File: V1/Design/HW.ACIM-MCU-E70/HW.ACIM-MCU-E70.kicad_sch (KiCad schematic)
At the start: 35 parts, among them J1 HEADER 2x15POS, J2 HEADER 2x15POS, U1 ATSAME70J20B, U2 12MHz

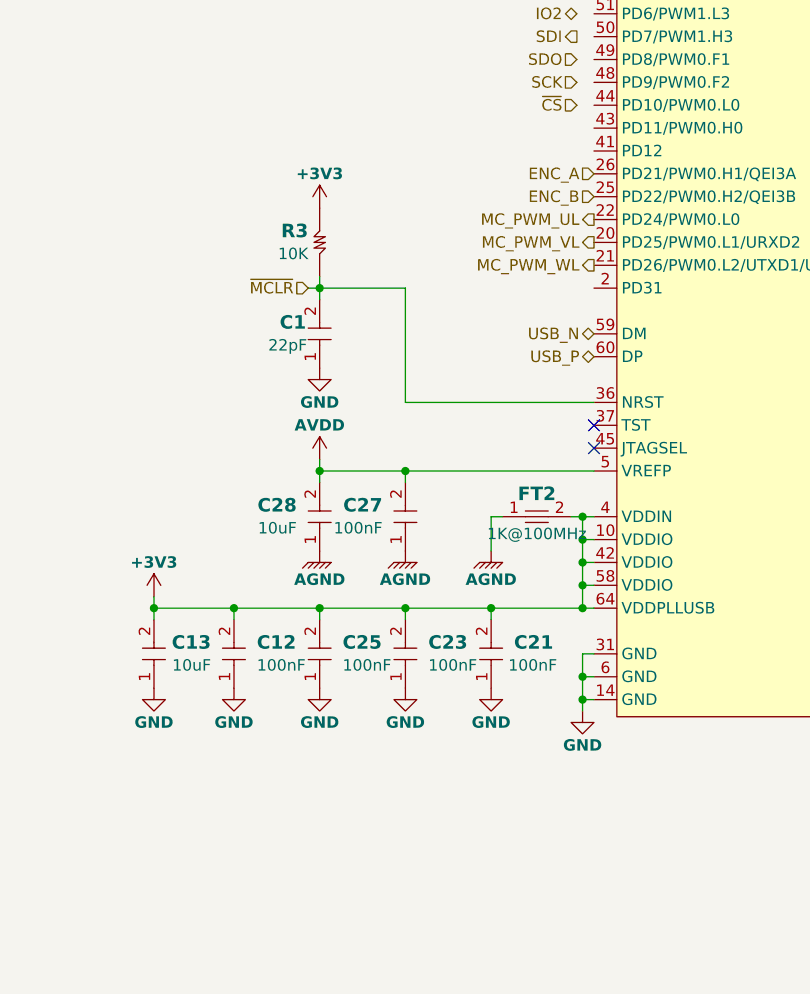
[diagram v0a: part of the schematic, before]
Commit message: HW.ACIM-MCU-E70 schematic update 2
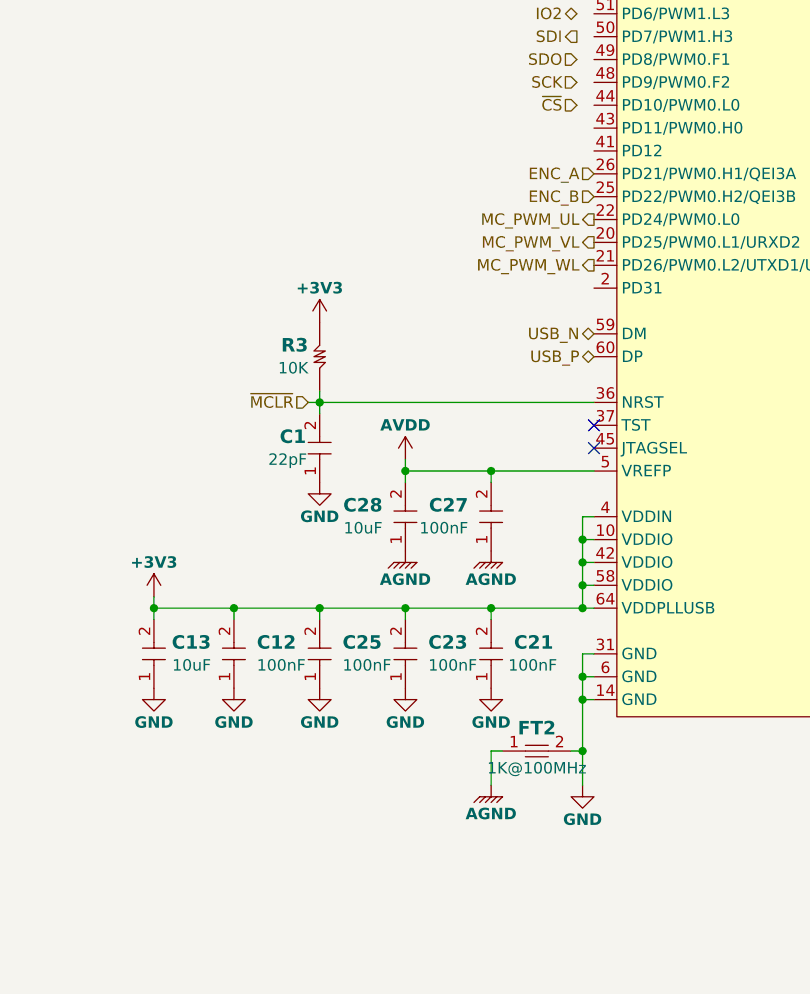
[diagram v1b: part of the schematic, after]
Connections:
- net +3V3: no longer FT2.2
- net GND: now also FT2.2
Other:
- moved on the sheet: C1, C27, C28, FT2, R3
